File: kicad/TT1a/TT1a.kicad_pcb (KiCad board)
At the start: 2 copper layers, 22 parts, among them SW1 SW_Push, SW2 SW_Push, SW3 SW_Push, SW4 SW_Push, U1 ATtiny404-SS

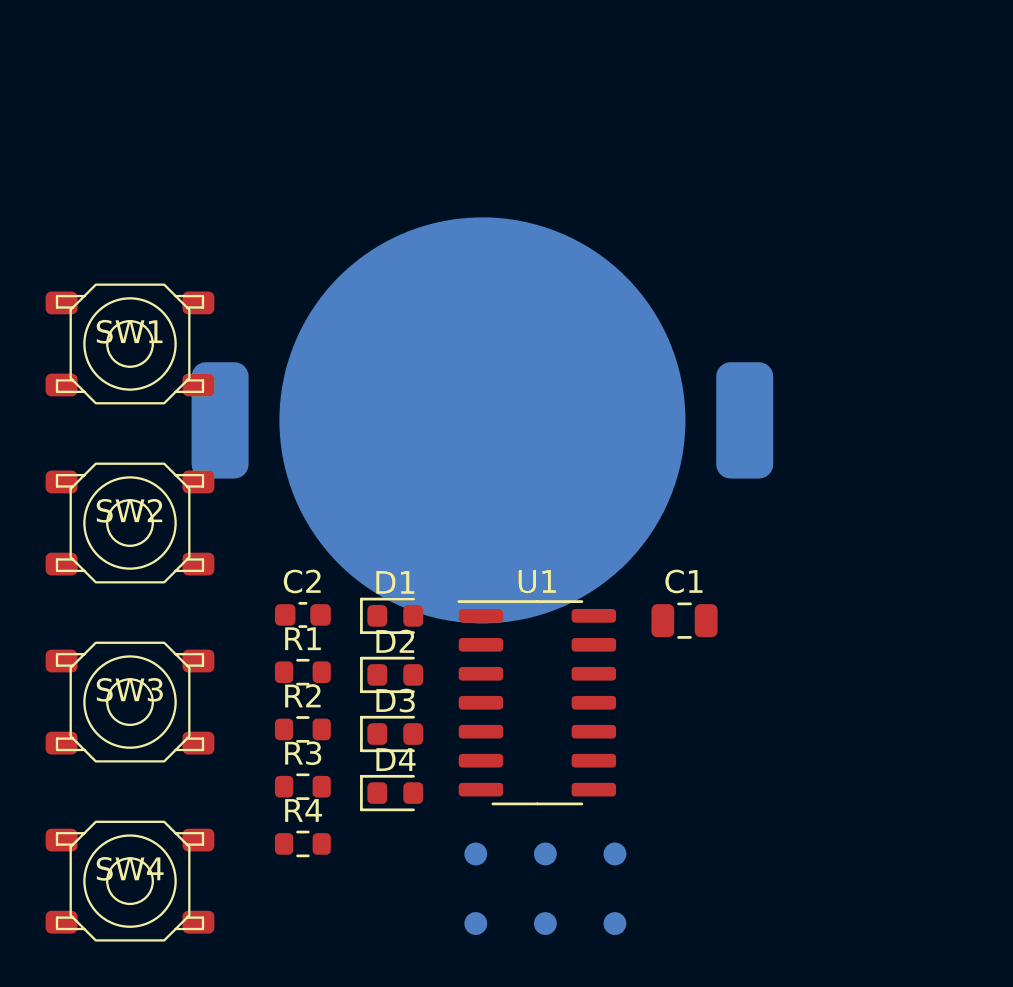
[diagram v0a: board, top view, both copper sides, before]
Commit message: pcb TT1a done
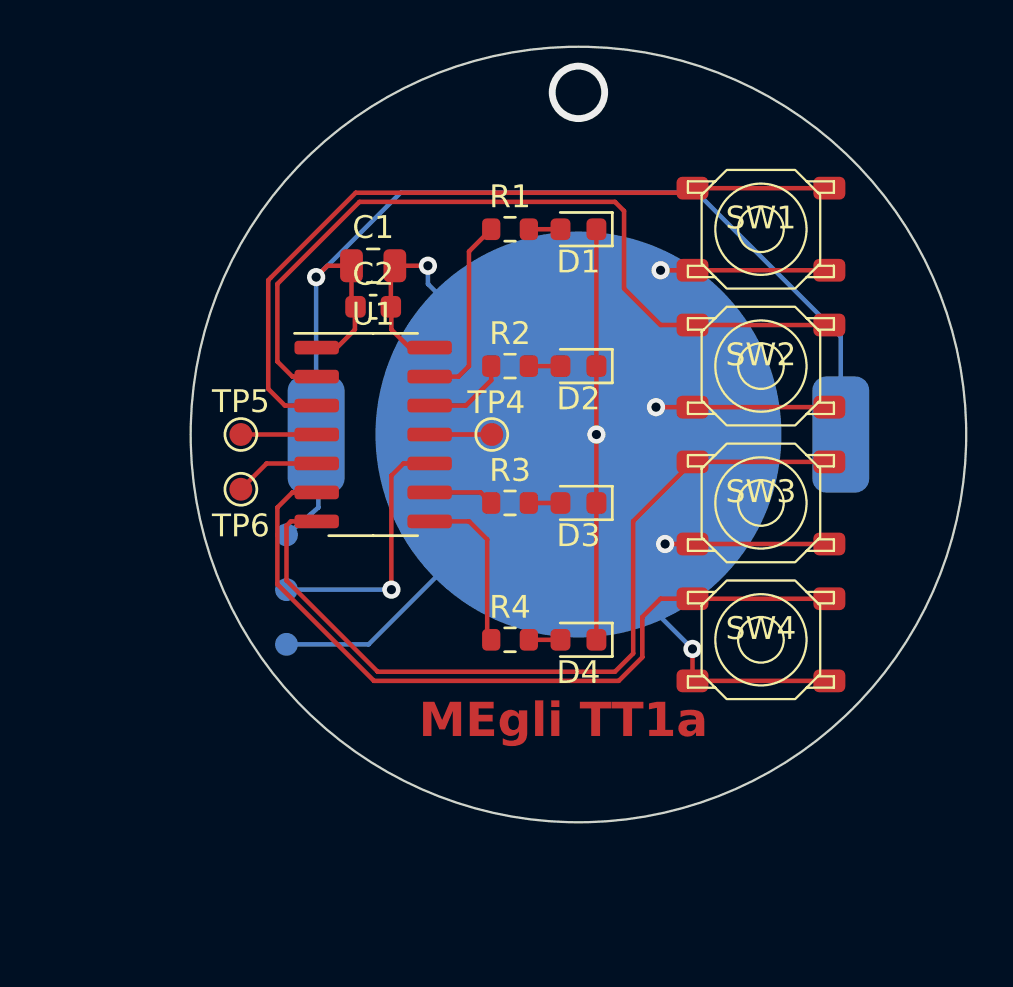
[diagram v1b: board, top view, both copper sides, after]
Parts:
- TP4, TP5, TP6: moved to F.Cu
- moved SW4 29.6 mm to (108.0, 79.0)
- moved SW3 29.0 mm to (108.0, 73.0)
- moved SW2 28.5 mm to (108.0, 67.0)
- moved SW1 28.1 mm to (108.0, 61.0)
- moved TP6 21.6 mm to (85.2, 72.4), turned to 0 degrees
- moved TP4 21.6 mm to (96.2, 70.0), turned to 0 degrees
- moved R1 21.4 mm to (97.0, 61.0)
- moved TP5 21.1 mm to (85.2, 70.0), turned to 0 degrees
- moved C1 20.7 mm to (91.0, 62.6)
- moved TP1 20.1 mm to (87.2, 74.4)
- moved TP2 18.9 mm to (87.2, 79.2)
- moved D1 18.8 mm to (100.0, 61.0), turned to 180 degrees
- moved R2 18.3 mm to (97.0, 67.0)
- moved TP3 16.2 mm to (87.2, 76.8)
- moved D2 15.7 mm to (100.0, 67.0), turned to 180 degrees
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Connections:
- TP5 pad 1: Net-(U1-PA2) -> Net-(U1-PA6)
- TP6 pad 1: Net-(U1-PA3) -> Net-(U1-PA7)
- U1 pad 12: Net-(U1-PA2) -> /LED2
- U1 pad 13: Net-(U1-PA3) -> /LED1
- U1 pad 2: /LED1 -> /BTN2
- U1 pad 3: /LED2 -> /BTN1
- U1 pad 4: /LED3 -> Net-(U1-PA6)
- U1 pad 5: /LED4 -> Net-(U1-PA7)
- U1 pad 8: /BTN2 -> /LED4
- U1 pad 9: /BTN1 -> /LED3
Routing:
- net GND: track 0.00 -> 98.5 mm, vias 0 -> 6
- net +BATT: track 0.00 -> 50.1 mm, vias 0 -> 1
- net /BTN3: track 0.00 -> 36.5 mm
- net /BTN2: track 0.00 -> 35.3 mm
- net /BTN4: track 0.00 -> 33.8 mm
- net /BTN1: track 0.00 -> 33.6 mm
- net Net-(U1-~{RESET}/PA0): track 0.00 -> 11.5 mm, vias 0 -> 1
- net /LED1: track 0.00 -> 8.32 mm
- net /LED4: track 0.00 -> 7.32 mm
- net Net-(U1-PA7): track 0.00 -> 3.79 mm
- net /LED2: track 0.00 -> 3.78 mm
- net Net-(U1-PA6): track 0.00 -> 3.33 mm
- net /LED3: track 0.00 -> 2.89 mm
- net Net-(U1-PA1): track 0.00 -> 2.73 mm
- net Net-(D4-A): track 0.00 -> 1.39 mm
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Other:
- board outline added: 34 x 34 mm
- board text added: "MEgli TT1a"
